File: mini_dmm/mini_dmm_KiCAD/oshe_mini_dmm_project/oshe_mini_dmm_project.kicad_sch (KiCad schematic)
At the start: 42 parts, among them J1 FTDI Basic, J2 ICSP, J3 DISPLAY, J4 TEST LEAD CONNECTIONS, SW1 PTS526 SK15 SMTR2 LFS, SW2 PTS526 SK15 SMTR2 LFS, SW3 SW_DPDT_x2, U1 LM324, U2 ATmega328P-A, U3 BU91796FS-ME2, U4 LM2664M6, Y1 16MHz

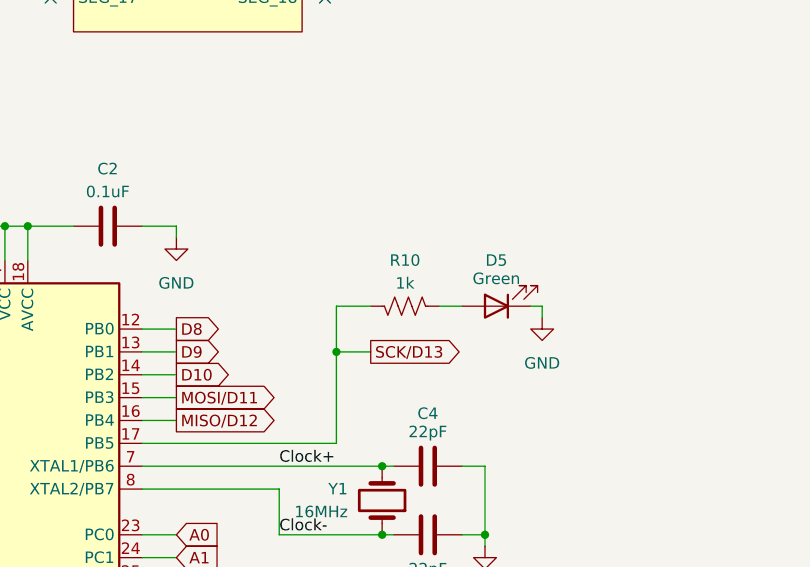
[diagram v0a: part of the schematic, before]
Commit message: Revert "Merge branch 'main' of https://github.com/peterk-mtu/oshe-dmm"
This reverts commit ce5d962f54be2277657b6d8c67a3a7c391f0a935, reversing
changes made to f95ec51989ec9ec0648d62f0b87f0342297760cd.
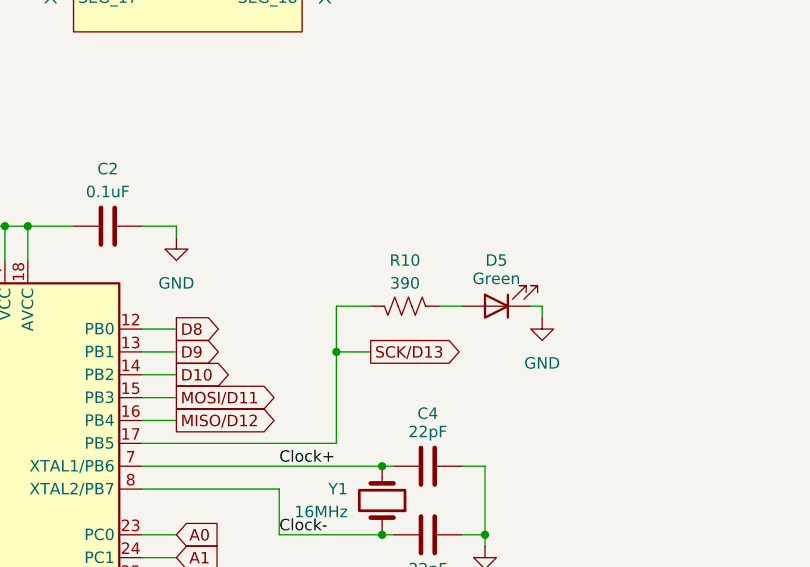
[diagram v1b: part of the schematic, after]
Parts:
- R10: value 1k -> 390
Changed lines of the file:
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@@
 			)
 		)
-		(property "Value" "1k"
+		(property "Value" "390"
 			(at 246.38 100.33 90)
 			(effects
